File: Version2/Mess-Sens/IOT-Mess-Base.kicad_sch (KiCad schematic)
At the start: 43 parts, among them IC1 SHT40I-AD1F-R2, J1 Conn_01x06_Pin, J2 Conn_01x04_Pin, J3 Jumper_2, J4 Conn_01x04_Pin, J5 Jumper_2, J6 Conn_01x02_Pin, J7 Jumper_2, J8 Conn_01x02_Pin, U1 LTR-303/308, U10 ENS210, U11 MTS4 0.1C DFN-4L, U12 T117W 0.1C DFN-6L, U13 QMC6309/WLCSP-4, U14 SHT31-DIS, U15 TMP102xxDRL 0.5C SOT-563, U16 DS1307Z+, U2 LTR-507ALS, U3 INA219AxDCN, U4 USB_C_Receptacle_USB2.0_16P, U5 BH1750FVI-TR, U6 APDS-9960, U7 MMC5633NJL/WLP-4, U8 ME6211C33M5, U9 HDC2010/DSBGA-6

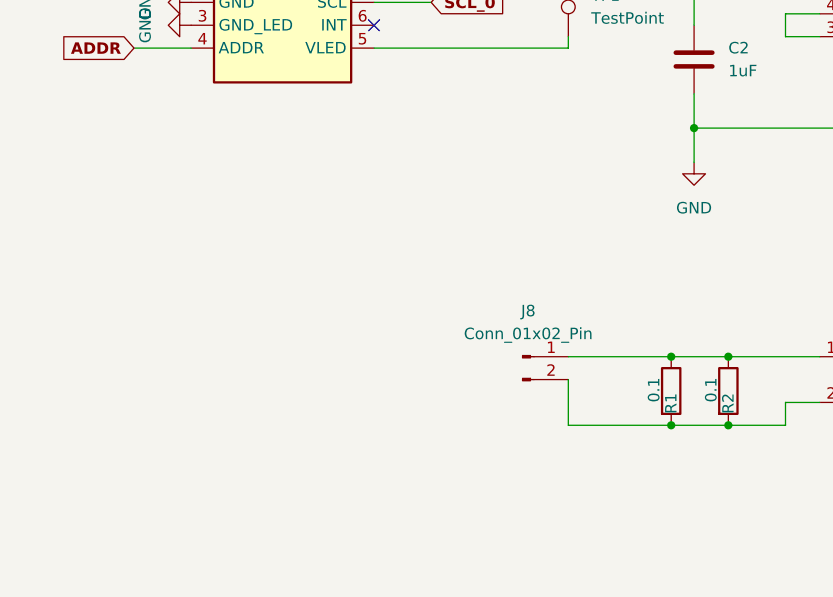
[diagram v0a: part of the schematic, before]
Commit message: update.
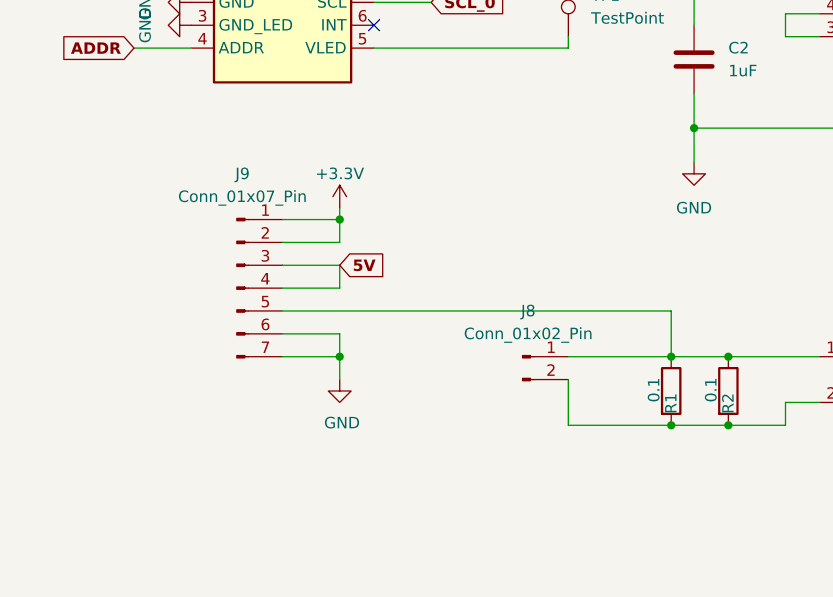
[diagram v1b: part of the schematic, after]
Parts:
- added J9: Conn_01x07_Pin, Connector_PinHeader_2.54mm:PinHeader_1x07_P2.54mm_Vertical, symbol Connector:Conn_01x07_Pin
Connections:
- net +3.3V: now also J9.1 (Pin_1), J9.2 (Pin_2)
- net 5V: now also J9.3 (Pin_3), J9.4 (Pin_4)
- net GND: now also J9.6 (Pin_6), J9.7 (Pin_7)
- net at J8.1 (Pin_1), R1.1, R2.1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: now also J9.5 (Pin_5)

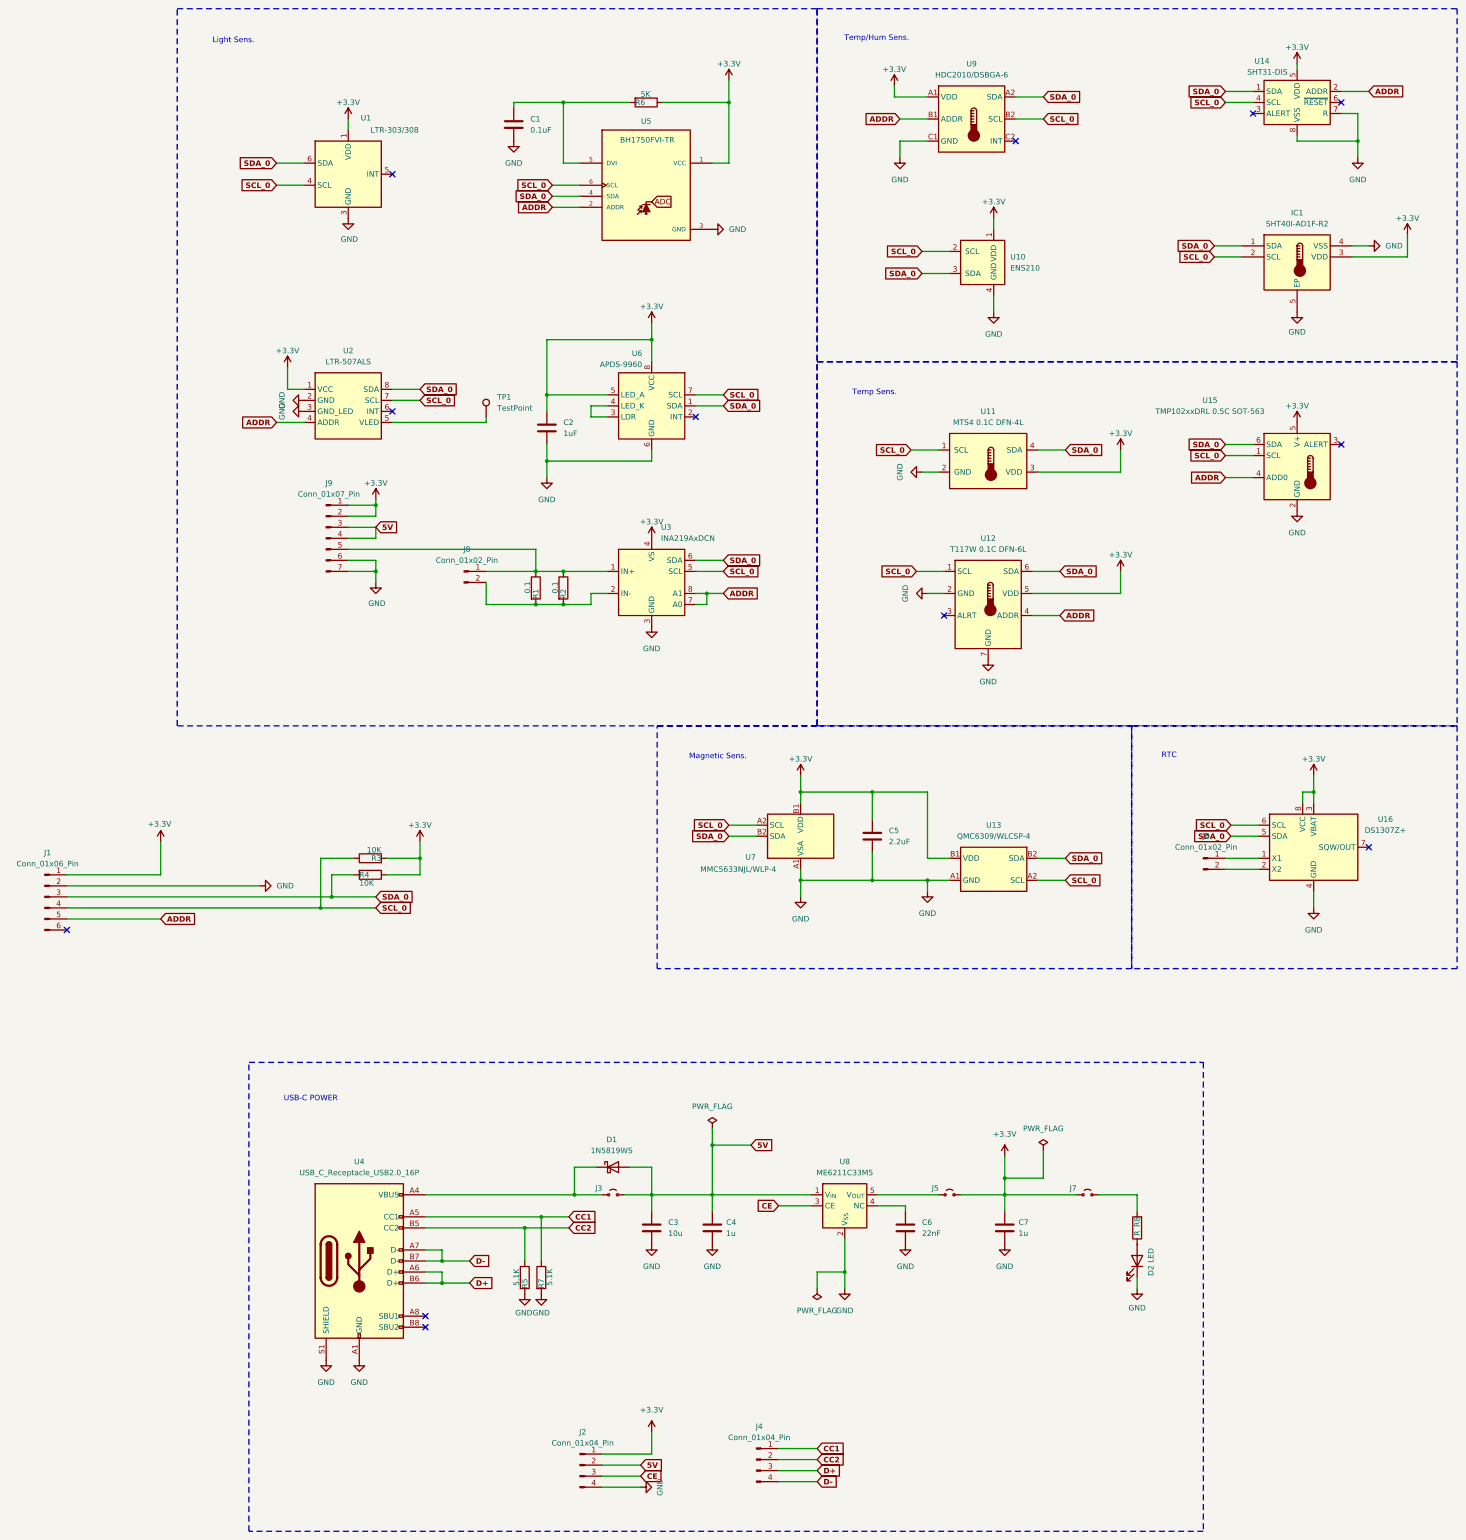
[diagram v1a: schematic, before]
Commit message: update.
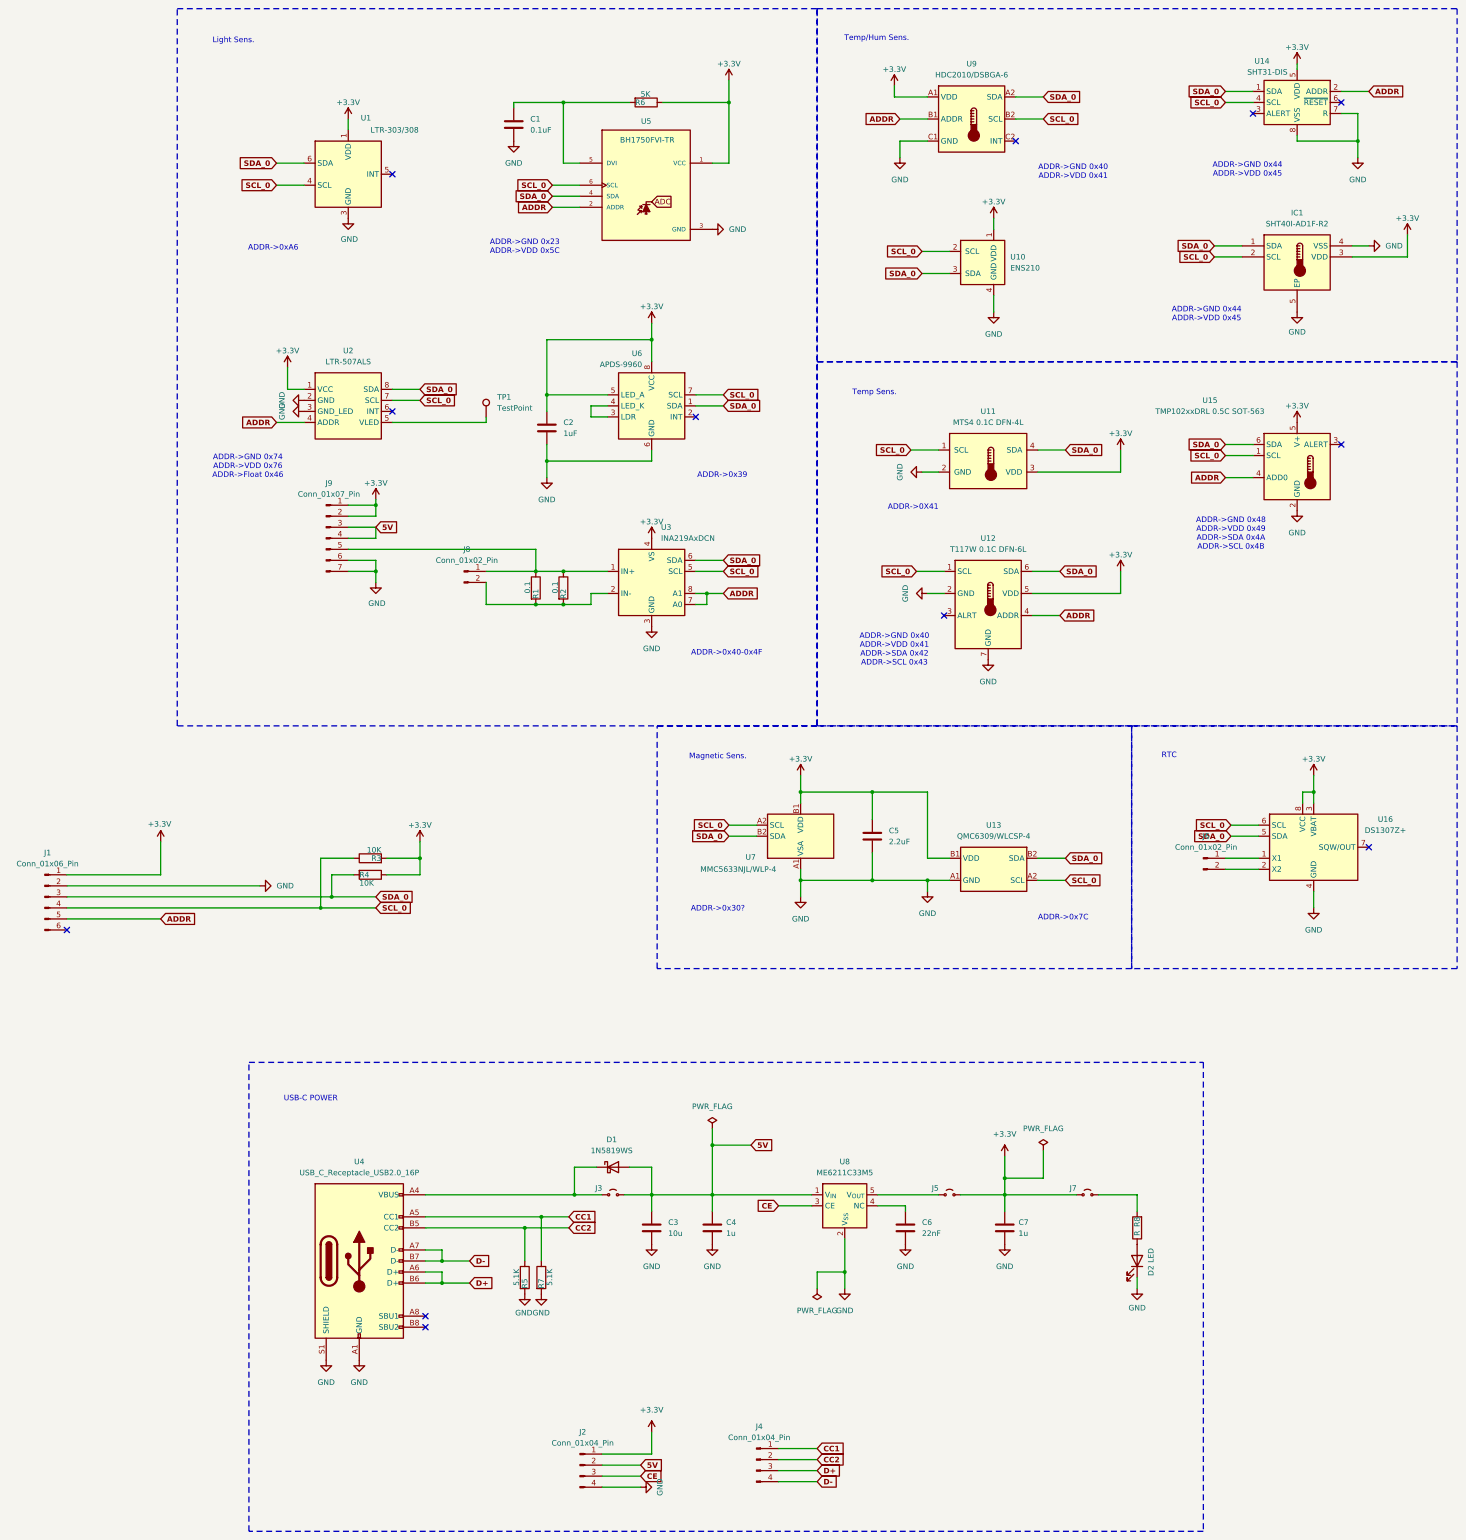
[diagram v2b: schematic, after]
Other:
- note added: "ADDR->0X41"
- note added: "ADDR->0x30?"
- note added: "ADDR->0x39"
- note added: "ADDR->0x40-0x4F"
- note added: "ADDR->0x7C"
- note added: "ADDR->0xA6"
- note added: "ADDR->GND 0x23 ADDR->VDD 0x5C"
- note added: "ADDR->GND 0x40 ADDR->VDD 0x41"
- note added: "ADDR->GND 0x40 ADDR->VDD 0x41 ADDR->SDA 0x42 ADDR->SCL 0x43"
- note added: "ADDR->GND 0x44 ADDR->VDD 0x45"
- note added: "ADDR->GND 0x48 ADDR->VDD 0x49 ADDR->SDA 0x4A ADDR->SCL 0x4B"
- note added: "ADDR->GND 0x74 ADDR->VDD 0x76 ADDR->Float 0x46"
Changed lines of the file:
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@@
 		)
 	)
+	(text "ADDR->0x40-0x4F"
+		(exclude_from_sim no)
+		(at 278.892 183.896 0)
+		(effects
+			(font
+				(size 1.27 1.27)
+			)
+		)
+	)
 	(text "USB-C POWER"
 		(exclude_from_sim no)
@@
 		)
 	)
+	(text "ADDR->GND 0x40\nADDR->VDD 0x41"
+		(exclude_from_sim no)
+		(at 358.648 73.152 0)
+		(effects
+			(font
+				(size 1.27 1.27)
+			)
+		)
+	)
+	(text "ADDR->GND 0x48\nADDR->VDD 0x49\nADDR->SDA 0x4A\nADDR->SCL 0x4B"
+		(exclude_from_sim no)
+		(at 394.97 156.464 0)
+		(effects
+			(font
+				(size 1.27 1.27)
+			)
+		)
+	)
+	(text "ADDR->0x39"
+		(exclude_from_sim no)
+		(at 277.876 143.002 0)
+		(effects
+			(font
+				(size 1.27 1.27)
+			)
+		)
+	)
+	(text "ADDR->GND 0x44\nADDR->VDD 0x45"
+		(exclude_from_sim no)
+		(at 398.78 72.644 0)
+		(effects
+			(font
+				(size 1.27 1.27)
+			)
+		)
+	)
+	(text "ADDR->0x7C"
+		(exclude_from_sim no)
+		(at 356.362 244.856 0)
+		(effects
+			(font
+				(size 1.27 1.27)
+			)
+		)
+	)
 	(text "Temp Sens."
 		(exclude_from_sim no)
@@
 		)
 	)
+	(text "ADDR->0X41\n"
+		(exclude_from_sim no)
+		(at 321.818 150.368 0)
+		(effects
+			(font
+				(size 1.27 1.27)
+			)
+		)
+	)
+	(text "ADDR->GND 0x44\nADDR->VDD 0x45"
+		(exclude_from_sim no)
+		(at 389.382 105.918 0)
+		(effects
+			(font
+				(size 1.27 1.27)
+			)
+		)
+	)
+	(text "ADDR->GND 0x40\nADDR->VDD 0x41\nADDR->SDA 0x42\nADDR->SCL 0x43"
+		(exclude_from_sim no)
+		(at 317.5 183.134 0)
+		(effects
+			(font
+				(size 1.27 1.27)
+			)
+		)
+	)
+	(text "ADDR->0xA6"
+		(exclude_from_sim no)
+		(at 174.498 90.678 0)
+		(effects
+			(font
+				(size 1.27 1.27)
+			)
+		)
+	)
 	(text "Magnetic Sens."
 		(exclude_from_sim no)
@@
 		)
 	)
+	(text "ADDR->0x30?"
+		(exclude_from_sim no)
+		(at 276.86 242.824 0)
+		(effects
+			(font
+				(size 1.27 1.27)
+			)
+		)
+	)
 	(text "Temp/Hum Sens."
 		(exclude_from_sim no)
@@
 		)
 	)
+	(text "ADDR->GND 0x23\nADDR->VDD 0x5C"
+		(exclude_from_sim no)
+		(at 232.41 90.424 0)
+		(effects
+			(font
+				(size 1.27 1.27)
+			)
+		)
+	)
+	(text "ADDR->GND 0x74\nADDR->VDD 0x76\nADDR->Float 0x46"
+		(exclude_from_sim no)
+		(at 168.656 140.97 0)
+		(effects
+			(font
+				(size 1.27 1.27)
+			)
+		)
+	)
 	(junction
 		(at 185.42 242.57)
@@
 			)
 		)
-		(property "Datasheet" ""
+		(property "Datasheet" "https://optoelectronics.liteon.com/upload/download/DS86-2013-0014/LTR-507ALS-01_FINAL%20DS.pdf"
 			(at 191.77 116.84 0)
 			(effects
@@
 			)
 		)
-		(property "Datasheet" "https://www.sensirion.com/fileadmin/user_upload/customers/sensirion/Dokumente/2_Humidity_Sensors/Datasheets/Sensirion_Humidity_Sensors_SHT3x_Datasheet_digital.pdf"
+		(property "Datasheet" "https://sensirion.com/media/documents/213E6A3B/63A5A569/Datasheet_SHT3x_DIS.pdf"
 			(at 410.21 55.88 0)
 			(effects
